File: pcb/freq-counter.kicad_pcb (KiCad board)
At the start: 4 copper layers, 152.4 x 190.5 mm, 103 parts, among them J1 RPM on board, J10 Power_T1, J2 BNC, J3 RPM to Board, J4 Jack-DC, J5 Segments-Terminal0, J6 Digits-Terminal0, J7 Segments-Terminal1, J8 Digits-Terminal1, J9 Power_Terminal1, Q1 CSC388A, Q10 2SC1815, Q11 2SC1815, Q12 2SC1815, Q13 2SC1815, Q14 2SC1815, Q2 CSC388A, Q3 2SA1015, Q4 2SC1815, Q5 2SC1815, Q6 CSC388A, Q7 CSC388A, Q8 CSC388A, Q9 2SC1815, SW1 on/off, SW2 count up, SW3 toggle, SW4 SW_SIGNAL, U1 SN74HC02N, U2 ATTINY4313-PU(freq-counter), U3 EE-SX460, U4 74HC00, U5 74HC00, U6 74HC00, U7 7seg-2digit-ca, U8 7seg-2digit-ca, U9 7seg-2digit-ca, Y1 10MHz

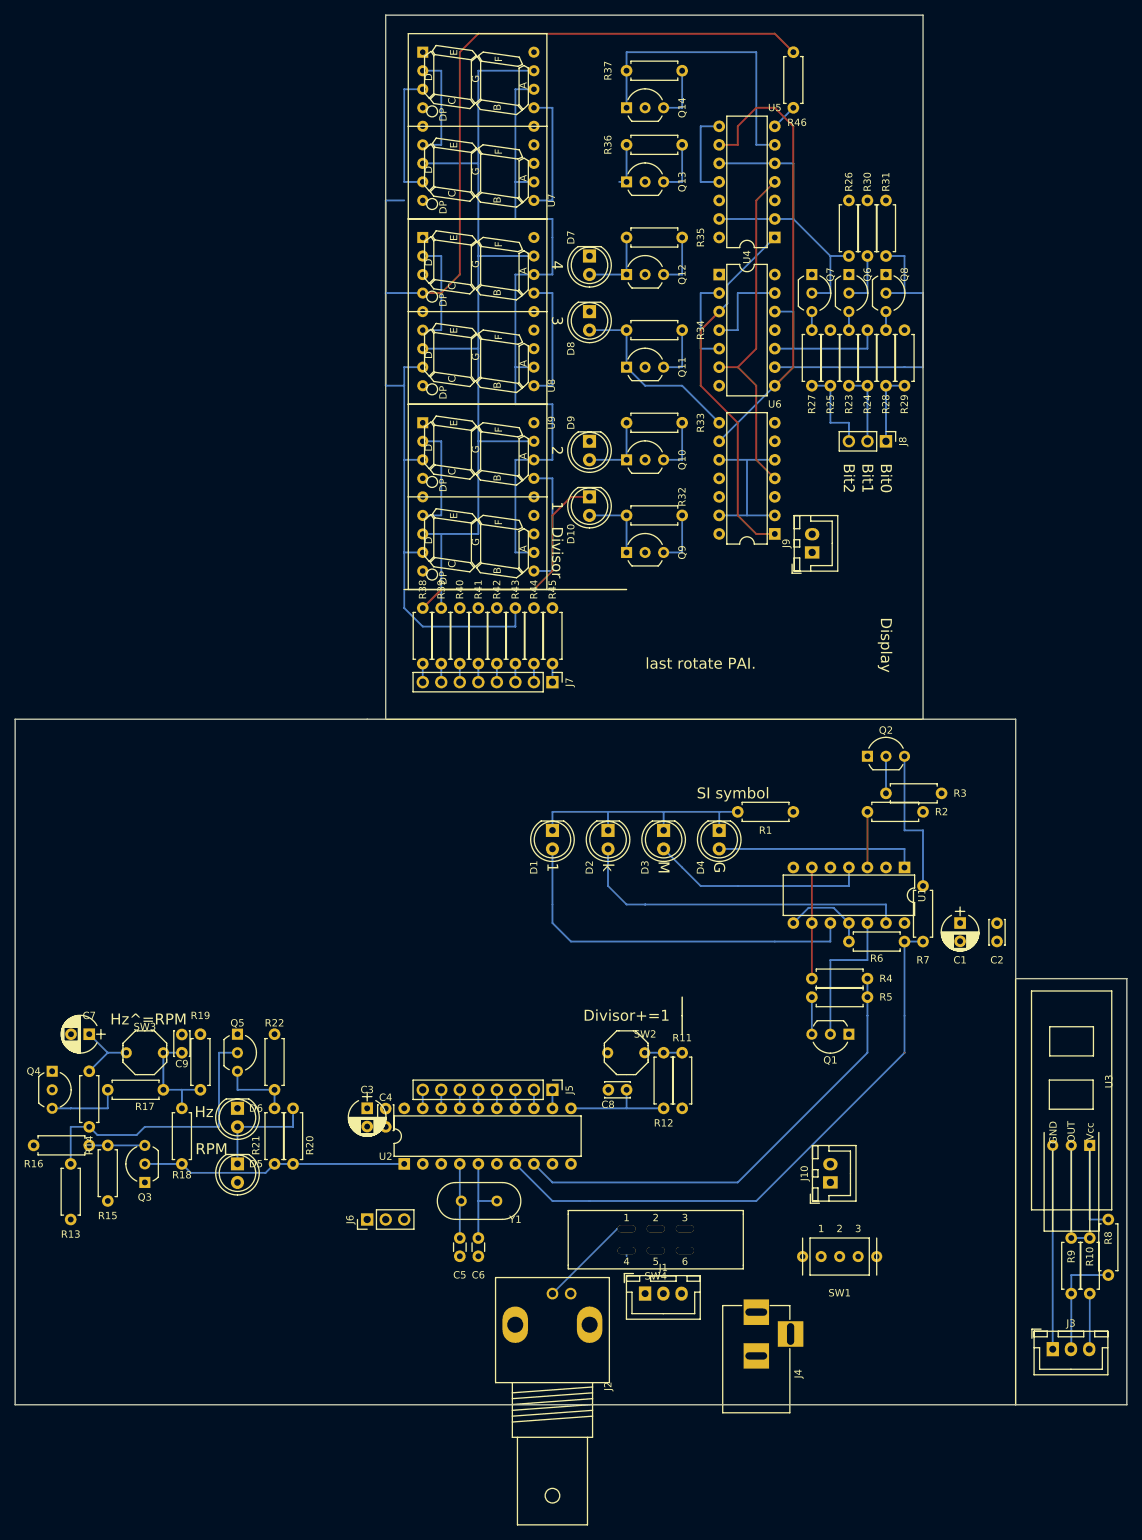
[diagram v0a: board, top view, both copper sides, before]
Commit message: Display板の大きさ，向きが決まった。Displayに合わせて母板を仕上げる。
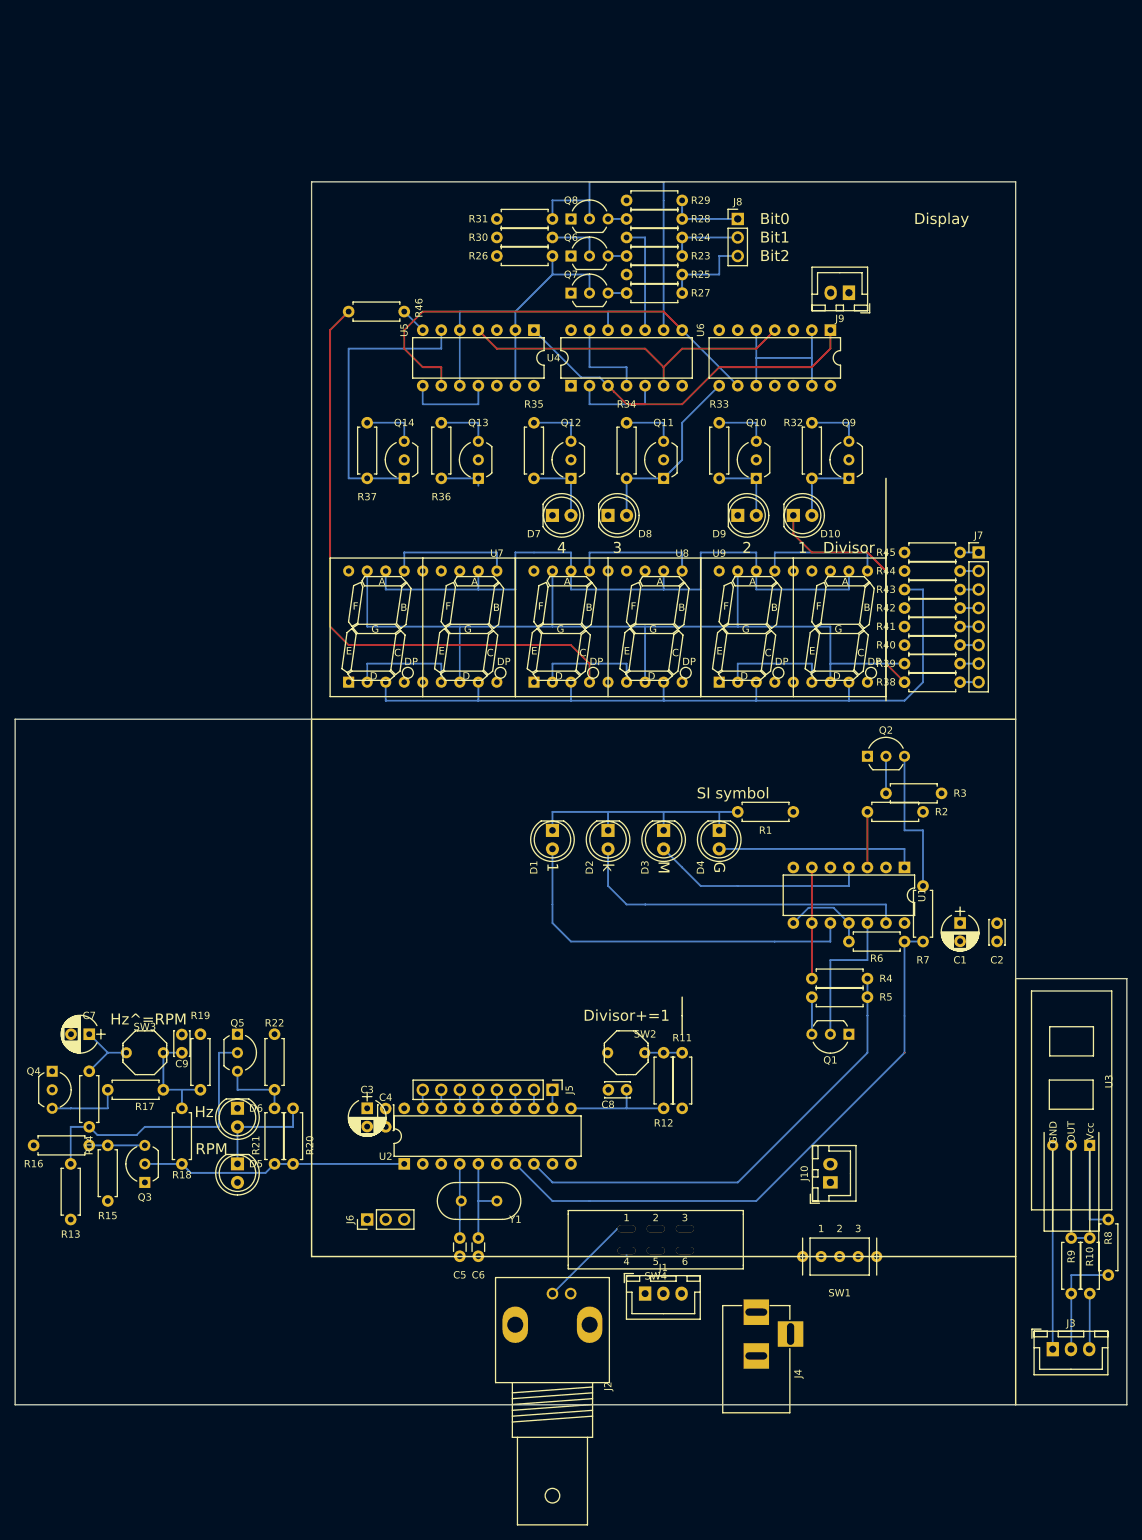
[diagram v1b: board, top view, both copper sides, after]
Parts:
- moved U7 69.1 mm to (99.1, 91.6), turned to 0 degrees
- moved R38 66.8 mm to (165.1, 99.1), turned to 0 degrees
- moved R37 64.8 mm to (91.4, 63.5), turned to 270 degrees
- moved R39 64.0 mm to (165.1, 96.5), turned to 0 degrees
- moved R40 61.2 mm to (165.1, 94.0), turned to 0 degrees
- moved J7 61.1 mm to (175.3, 81.3), turned to 0 degrees
- moved R46 60.2 mm to (96.5, 48.3), turned to 180 degrees
- moved Q14 59.2 mm to (96.5, 71.1), turned to 90 degrees
- moved R41 58.5 mm to (165.1, 91.4), turned to 0 degrees
- moved R42 55.9 mm to (165.1, 88.9), turned to 0 degrees
- moved R43 53.4 mm to (165.1, 86.4), turned to 0 degrees
- moved R44 51.1 mm to (165.1, 83.8), turned to 0 degrees
- moved R36 50.4 mm to (101.6, 63.5), turned to 270 degrees
- moved R45 48.9 mm to (165.1, 81.3), turned to 0 degrees
- moved U9 46.9 mm to (149.9, 91.6), turned to 0 degrees
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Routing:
- net /7seg/KC: track 113.3 -> 105.7 mm
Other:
- board size 152.4 x 190.5 mm -> 152.4 x 167.6 mm
- board text removed: "last rotate PAI."
